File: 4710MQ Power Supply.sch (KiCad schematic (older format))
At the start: 26 parts, among them J1 Jack-DC, J2 ATX 4 Pin, J3 Molex 4 Pin, J4 USB_B_Micro, U1 MP1499GD-Z, U2 CH340G, U3 LM1117-3.3, U4 ACS716xLATR-12BB-NL, U5 TSM1285BCSA

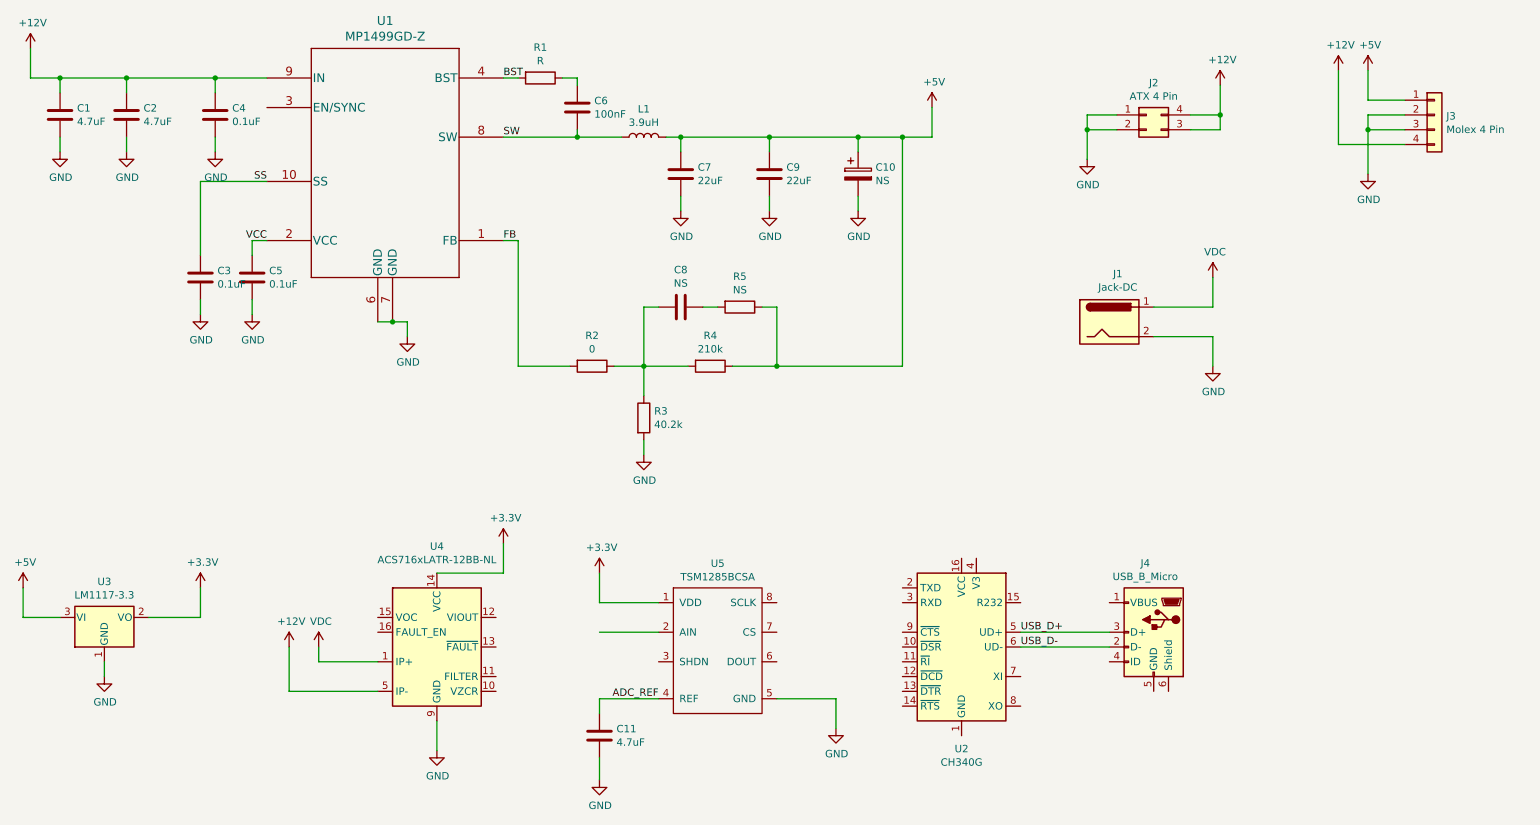
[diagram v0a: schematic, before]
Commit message: Version 2.0
- Size Changed
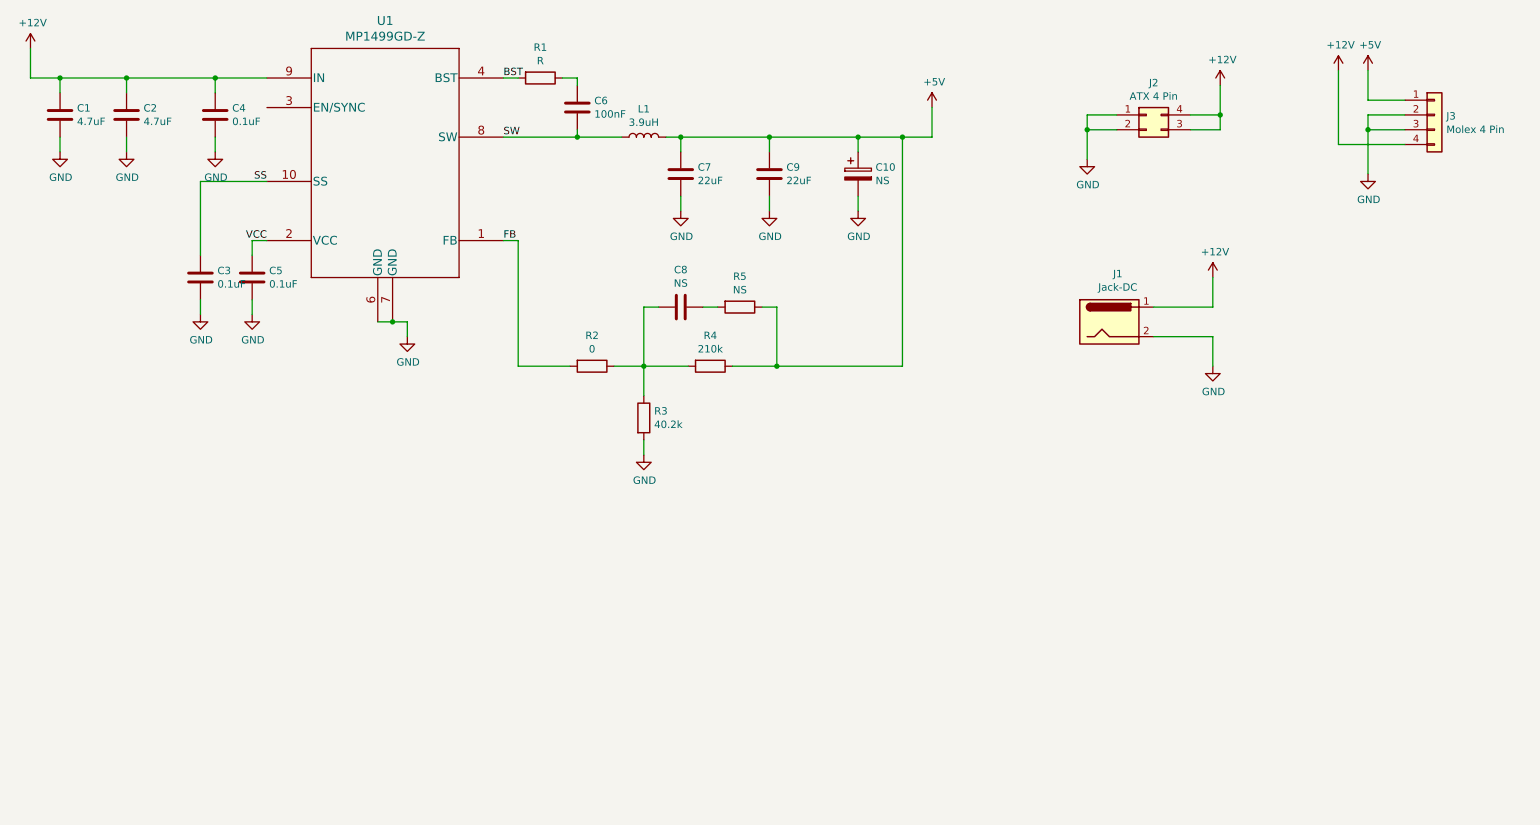
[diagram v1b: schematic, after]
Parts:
- removed C11: 4.7uF, Capacitor_SMD:C_1206_3216Metric_Pad1.33x1.80mm_HandSolder, symbol Device:C
- removed J4: USB_B_Micro, Connector_USB:USB_Micro-B_Wuerth_614105150721_Vertical, symbol Connector:USB_B_Micro
- removed U2: CH340G, Package_SO:SOIC-16_3.9x9.9mm_P1.27mm, symbol Interface_USB:CH340G
- removed U3: LM1117-3.3, Package_TO_SOT_SMD:SOT-23_Handsoldering, symbol Regulator_Linear:LM1117-3.3
- removed U4: ACS716xLATR-12BB-NL, Package_SO:SOIC-16W_7.5x10.3mm_P1.27mm, symbol Sensor_Current:ACS716xLATR-12BB-NL
- removed U5: TSM1285BCSA, Package_SO:SOIC-8_3.9x4.9mm_P1.27mm, symbol TSM1285BCSA:TSM1285BCSA
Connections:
- net VDC is gone; now on net +12V: J1.1
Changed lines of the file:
@@
 Wire Wire Line
 	4850 3650 4850 3750
-$Comp
-L power:GND #PWR010
-U 1 1 611AF7F5
-P 4850 3750
-F 0 "#PWR010" H 4850 3500 50  0001 C CNN
-F 1 "GND" H 4855 3577 50  0000 C CNN
-F 2 "" H 4850 3750 50  0001 C CNN
-F 3 "" H 4850 3750 50  0001 C CNN
-	1    4850 3750
-	1    0    0    -1
-$EndComp
 Wire Wire Line
 	4000 3150 4350 3150
@@
 $EndComp
 $Comp
-L power:VDC #PWR0112
-U 1 1 613D046F
+L power:+12V #PWR0101
+U 1 1 614C8ABC
 P 8700 2550
-F 0 "#PWR0112" H 8700 2450 50  0001 C CNN
-F 1 "VDC" H 8715 2723 50  0000 C CNN
+F 0 "#PWR0101" H 8700 2400 50  0001 C CNN
+F 1 "+12V" H 8715 2723 50  0000 C CNN
 F 2 "" H 8700 2550 50  0001 C CNN
 F 3 "" H 8700 2550 50  0001 C CNN
@@
 	1    0    0    -1
 $EndComp
-Text Label 4950 5400 2    50   ~ 0
-ADC_REF
-Text Label 7400 5050 0    50   ~ 0
-USB_D-
-Text Label 7400 4950 0    50   ~ 0
-USB_D+
-Wire Wire Line
-	7400 5050 8000 5050
-Wire Wire Line
-	7400 4950 8000 4950
-$Comp
-L power:GND #PWR0108
-U 1 1 61468F1F
-P 6150 5600
-F 0 "#PWR0108" H 6150 5350 50  0001 C CNN
-F 1 "GND" H 6155 5427 50  0000 C CNN
-F 2 "" H 6150 5600 50  0001 C CNN
-F 3 "" H 6150 5600 50  0001 C CNN
-	1    6150 5600
-	1    0    0    -1
-$EndComp
-Wire Wire Line
-	6150 5400 6150 5600
-Wire Wire Line
-	5750 5400 6150 5400
-$Comp
-L power:GND #PWR0107
-U 1 1 61465E71
-P 4550 5950
-F 0 "#PWR0107" H 4550 5700 50  0001 C CNN
-F 1 "GND" H 4555 5777 50  0000 C CNN
-F 2 "" H 4550 5950 50  0001 C CNN
-F 3 "" H 4550 5950 50  0001 C CNN
-	1    4550 5950
-	1    0    0    -1
-$EndComp
-Wire Wire Line
-	4550 5800 4550 5950
-$Comp
-L Device:C C11
-U 1 1 61463231
-P 4550 5650
-F 0 "C11" H 4665 5696 50  0000 L CNN
-F 1 "4.7uF" H 4665 5605 50  0000 L CNN
-F 2 "Capacitor_SMD:C_1206_3216Metric_Pad1.33x1.80mm_HandSolder" H 4588 5500 50  0001 C CNN
-F 3 "~" H 4550 5650 50  0001 C CNN
-	1    4550 5650
-	1    0    0    -1
-$EndComp
-Wire Wire Line
-	4550 5400 4550 5500
-Wire Wire Line
-	4950 5400 4550 5400
-Wire Wire Line
-	4950 4950 4550 4950
-$Comp
-L power:+3.3V #PWR0106
-U 1 1 6145DF78
-P 4550 4550
-F 0 "#PWR0106" H 4550 4400 50  0001 C CNN
-F 1 "+3.3V" H 4565 4723 50  0000 C CNN
-F 2 "" H 4550 4550 50  0001 C CNN
-F 3 "" H 4550 4550 50  0001 C CNN
-	1    4550 4550
-	1    0    0    -1
-$EndComp
-Wire Wire Line
-	4550 4750 4550 4550
-Wire Wire Line
-	4950 4750 4550 4750
-$Comp
-L TSM1285BCSA:TSM1285BCSA U5
-U 1 1 61458BA8
-P 5350 5050
-F 0 "U5" H 5350 5615 50  0000 C CNN
-F 1 "TSM1285BCSA" H 5350 5524 50  0000 C CNN
-F 2 "Package_SO:SOIC-8_3.9x4.9mm_P1.27mm" H 5100 5500 50  0001 C CNN
-F 3 "" H 5100 5500 50  0001 C CNN
-	1    5350 5050
-	1    0    0    -1
-$EndComp
-$Comp
-L Connector:USB_B_Micro J4
-U 1 1 614532CD
-P 8300 4950
-F 0 "J4" H 8357 5417 50  0000 C CNN
-F 1 "USB_B_Micro" H 8357 5326 50  0000 C CNN
-F 2 "Connector_USB:USB_Micro-B_Wuerth_614105150721_Vertical" H 8450 4900 50  0001 C CNN
-F 3 "~" H 8450 4900 50  0001 C CNN
-	1    8300 4950
-	-1   0    0    -1
-$EndComp
-$Comp
-L Interface_USB:CH340G U2
-U 1 1 61446B15
-P 7000 5050
-F 0 "U2" H 7000 4361 50  0000 C CNN
-F 1 "CH340G" H 7000 4270 50  0000 C CNN
-F 2 "Package_SO:SOIC-16_3.9x9.9mm_P1.27mm" H 7050 4500 50  0001 L CNN
-F 3 "http://www.datasheet5.com/pdf-local-2195953" H 6650 5850 50  0001 C CNN
-	1    7000 5050
-	-1   0    0    -1
-$EndComp
-$Comp
-L power:GND #PWR0105
-U 1 1 6142B99E
-P 3450 5750
-F 0 "#PWR0105" H 3450 5500 50  0001 C CNN
-F 1 "GND" H 3455 5577 50  0000 C CNN
-F 2 "" H 3450 5750 50  0001 C CNN
-F 3 "" H 3450 5750 50  0001 C CNN
-	1    3450 5750
-	1    0    0    -1
-$EndComp
-Wire Wire Line
-	3450 5550 3450 5750
-$Comp
-L power:+3.3V #PWR0104
-U 1 1 61427B77
-P 3900 4350
-F 0 "#PWR0104" H 3900 4200 50  0001 C CNN
-F 1 "+3.3V" H 3915 4523 50  0000 C CNN
-F 2 "" H 3900 4350 50  0001 C CNN
-F 3 "" H 3900 4350 50  0001 C CNN
-	1    3900 4350
-	1    0    0    -1
-$EndComp
-Wire Wire Line
-	3900 4550 3900 4350
-Wire Wire Line
-	3450 4550 3900 4550
-Wire Wire Line
-	1500 4850 1850 4850
-$Comp
-L power:+3.3V #PWR0103
-U 1 1 6136B787
-P 1850 4650
-F 0 "#PWR0103" H 1850 4500 50  0001 C CNN
-F 1 "+3.3V" H 1865 4823 50  0000 C CNN
-F 2 "" H 1850 4650 50  0001 C CNN
-F 3 "" H 1850 4650 50  0001 C CNN
-	1    1850 4650
-	1    0    0    -1
-$EndComp
-Wire Wire Line
-	1850 4850 1850 4650
-Wire Wire Line
-	2450 5350 3050 5350
-$Comp
-L Sensor_Current:ACS716xLATR-12BB-NL U4
-U 1 1 613E1144
-P 3450 5050
-F 0 "U4" H 3450 5731 50  0000 C CNN
-F 1 "ACS716xLATR-12BB-NL" H 3450 5640 50  0000 C CNN
-F 2 "Package_SO:SOIC-16W_7.5x10.3mm_P1.27mm" H 3800 5000 50  0001 L CIN
-F 3 "http://www.allegromicro.com/~/media/Files/Datasheets/ACS716-Datasheet.ashx?la=en" H 3450 5050 50  0001 C CNN
-	1    3450 5050
-	1    0    0    -1
-$EndComp
-$Comp
-L power:+12V #PWR0114
-U 1 1 613D734C
-P 2450 5050
-F 0 "#PWR0114" H 2450 4900 50  0001 C CNN
-F 1 "+12V" H 2465 5223 50  0000 C CNN
-F 2 "" H 2450 5050 50  0001 C CNN
-F 3 "" H 2450 5050 50  0001 C CNN
-	1    2450 5050
-	1    0    0    -1
-$EndComp
-$Comp
-L power:VDC #PWR0113
-U 1 1 613D6C08
-P 2650 5050
-F 0 "#PWR0113" H 2650 4950 50  0001 C CNN
-F 1 "VDC" H 2665 5223 50  0000 C CNN
-F 2 "" H 2650 5050 50  0001 C CNN
-F 3 "" H 2650 5050 50  0001 C CNN
-	1    2650 5050
-	1    0    0    -1
-$EndComp
-Wire Wire Line
-	2450 5350 2450 5050
-Wire Wire Line
-	2650 5150 2650 5050
-Wire Wire Line
-	3050 5150 2650 5150
-$Comp
-L power:GND #PWR0102
-U 1 1 6136914D
-P 1200 5250
-F 0 "#PWR0102" H 1200 5000 50  0001 C CNN
-F 1 "GND" H 1205 5077 50  0000 C CNN
-F 2 "" H 1200 5250 50  0001 C CNN
-F 3 "" H 1200 5250 50  0001 C CNN
-	1    1200 5250
-	1    0    0    -1
-$EndComp
-$Comp
-L power:+5V #PWR0101
-U 1 1 61368ADC
-P 650 4650
-F 0 "#PWR0101" H 650 4500 50  0001 C CNN
-F 1 "+5V" H 665 4823 50  0000 C CNN
-F 2 "" H 650 4650 50  0001 C CNN
-F 3 "" H 650 4650 50  0001 C CNN
-	1    650  4650
-	1    0    0    -1
-$EndComp
-Wire Wire Line
-	1200 5150 1200 5250
-Wire Wire Line
-	650  4850 650  4650
-Wire Wire Line
-	900  4850 650  4850
-$Comp
-L Regulator_Linear:LM1117-3.3 U3
-U 1 1 61364B65
-P 1200 4850
-F 0 "U3" H 1200 5092 50  0000 C CNN
-F 1 "LM1117-3.3" H 1200 5001 50  0000 C CNN
-F 2 "Package_TO_SOT_SMD:SOT-23_Handsoldering" H 1200 4850 50  0001 C CNN
-F 3 "http://www.ti.com/lit/ds/symlink/lm1117.pdf" H 1200 4850 50  0001 C CNN
-	1    1200 4850
-	1    0    0    -1
-$EndComp
+$Comp
+L power:GND #PWR?
+U 1 1 614CA392
+P 4850 3750
+F 0 "#PWR?" H 4850 3500 50  0001 C CNN
+F 1 "GND" H 4855 3577 50  0000 C CNN
+F 2 "" H 4850 3750 50  0001 C CNN
+F 3 "" H 4850 3750 50  0001 C CNN
+	1    4850 3750
+	1    0    0    -1
+$EndComp
